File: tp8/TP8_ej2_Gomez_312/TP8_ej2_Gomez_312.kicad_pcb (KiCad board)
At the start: 2 copper layers, 50 x 40 mm, 32 parts, among them J1 Output - RL, J10 Vemisor, J11 Vemisor, J2 Power, J3 Input, J5 GND, J6 Vbase, J7 Vbase, J8 Vbase, J9 Vemisor, Q1 BC548C, Q2 BC547, Q3 BC548C

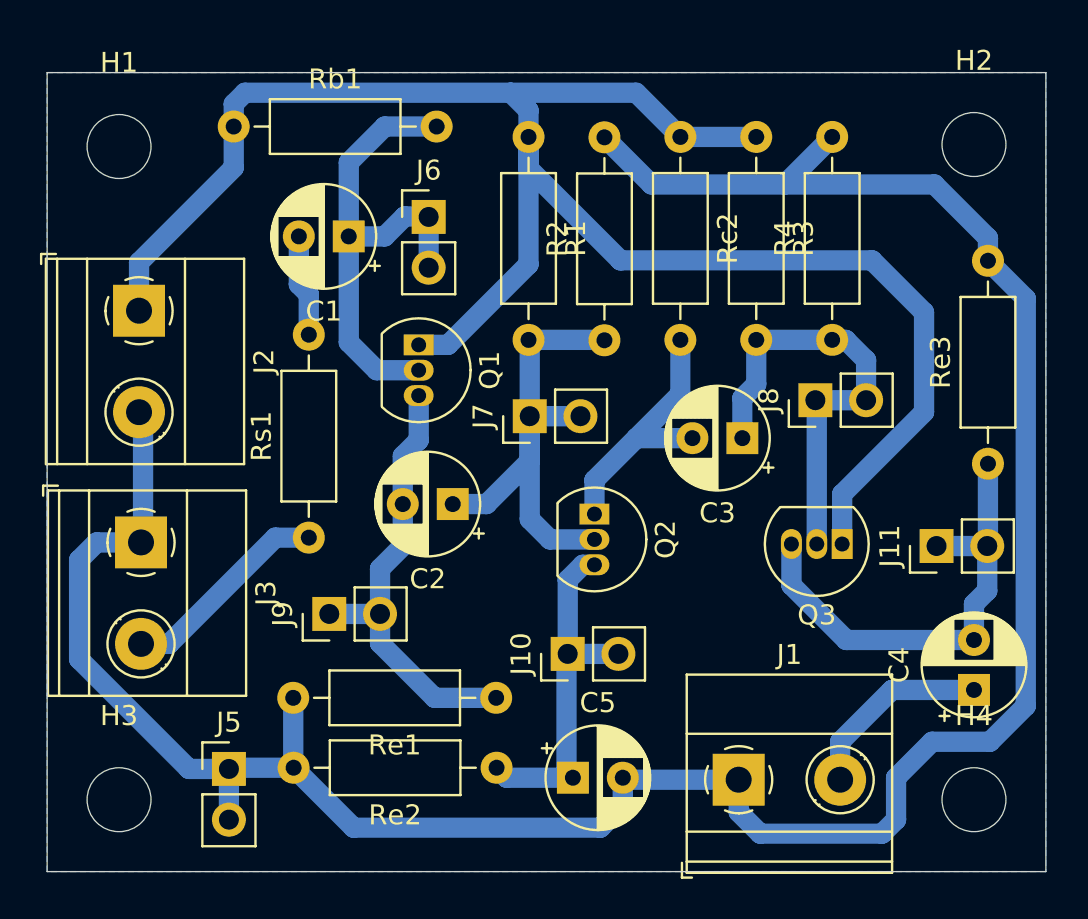
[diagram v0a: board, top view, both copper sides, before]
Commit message: finish tp8
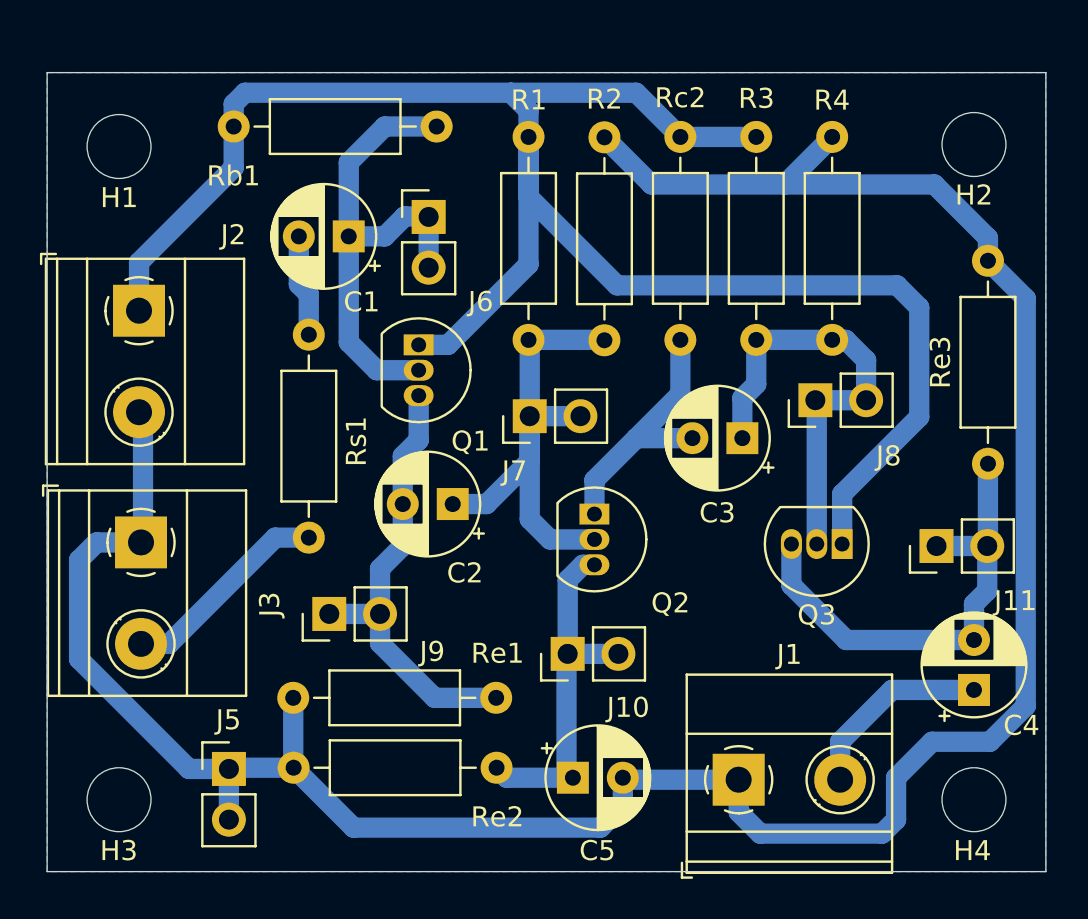
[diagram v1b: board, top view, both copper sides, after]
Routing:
- net VCC: track 93.4 -> 94.0 mm
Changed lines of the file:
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@@
 			(sketchpadsonfab no)
 			(subtractmaskfromsilk no)
-			(outputformat 1)
-			(mirror no)
-			(drillshape 1)
+			(outputformat 4)
+			(mirror yes)
+			(drillshape 0)
 			(scaleselection 1)
 			(outputdirectory "")
@@
 		(tags "Through hole pin header THT 1x02 2.54mm single row")
 		(property "Reference" "J7"
-			(at 0 -2.33 -90)
+			(at -2.75 -0.76 0)
 			(layer "F.SilkS")
 			(effects
@@
 		(tags "Through hole pin header THT 1x02 2.54mm single row")
 		(property "Reference" "J8"
-			(at 0 -2.33 270)
+			(at -2.8 3.67 0)
 			(layer "F.SilkS")
 			(effects
@@
 		)
 		(property "Value" "Vbase"
-			(at 0 4.87 270)
+			(at 0 4.87 -90)
 			(layer "F.Fab")
 			(effects
@@
 		)
 		(fp_text user "${REFERENCE}"
-			(at 0 1.27 360)
+			(at 0 1.27 0)
 			(layer "F.Fab")
 			(effects
@@
 		(tags "Resistor Axial_DIN0207 series Axial Horizontal pin pitch 10.16mm 0.25W = 1/4W length 6.3mm diameter 2.5mm")
 		(property "Reference" "R2"
-			(at 5.08 -2.37 -90)
+			(at 12.06 0 0)
 			(layer "F.SilkS")
 			(effects
@@
 		(tags "Resistor Axial_DIN0207 series Axial Horizontal pin pitch 10.16mm 0.25W = 1/4W length 6.3mm diameter 2.5mm")
 		(property "Reference" "Rs1"
-			(at 5.08 -2.37 -90)
+			(at 4.82 2.39 -90)
 			(layer "F.SilkS")
 			(effects
@@
 		(tags "Through hole pin header THT 1x02 2.54mm single row")
 		(property "Reference" "J11"
-			(at 0 -2.33 -90)
+			(at -2.75 3.955 0)
 			(layer "F.SilkS")
 			(effects
@@
 		(tags "Through hole pin header THT 1x02 2.54mm single row")
 		(property "Reference" "J10"
-			(at 0 -2.33 -90)
+			(at -2.69 3.03 0)
 			(layer "F.SilkS")
 			(effects
@@
 		(tags "Through hole pin header THT 1x02 2.54mm single row")
 		(property "Reference" "J9"
-			(at 0 -2.33 -90)
+			(at -1.89 5.155 0)
 			(layer "F.SilkS")
 			(effects
@@
 		(tags "mounting hole 3.2mm no annular m3")
 		(property "Reference" "H4"
-			(at 0 -4.2 0)
+			(at -0.08 2.56 0)
 			(layer "F.SilkS")
 			(effects
@@
 		(tags "Resistor Axial_DIN0207 series Axial Horizontal pin pitch 10.16mm 0.25W = 1/4W length 6.3mm diameter 2.5mm")
 		(property "Reference" "Rc2"
-			(at 5.08 -2.37 90)
+			(at -1.95 0 180)
 			(layer "F.SilkS")
 			(effects
@@
 		(tags "CP Radial series Radial pin pitch 2.50mm  diameter 5mm Electrolytic Capacitor")
 		(property "Reference" "C2"
-			(at 1.25 -3.75 180)
+			(at -0.614887 -3.46 180)
 			(layer "F.SilkS")
 			(effects
@@
 		(tags "THT Terminal Block Phoenix MKDS-1,5-2-5.08 pitch 5.08mm size 10.2x9.8mm^2 drill 1.3mm pad 2.6mm")
 		(property "Reference" "J3"
-			(at 2.54 -6.26 -90)
+			(at 3.1 -6.45 -90)
 			(layer "F.SilkS")
 			(effects
@@
 		(tags "Resistor Axial_DIN0207 series Axial Horizontal pin pitch 10.16mm 0.25W = 1/4W length 6.3mm diameter 2.5mm")
 		(property "Reference" "R3"
-			(at 5.08 -2.37 90)
+			(at -1.92 -0.01 180)
 			(layer "F.SilkS")
 			(effects
@@
 		(tags "to-92 sc-43 sc-43a sot54 PA33 transistor")
 		(property "Reference" "Q2"
-			(at 1.27 -3.56 90)
+			(at 4.46 -3.81 180)
 			(layer "F.SilkS")
 			(effects
@@
 		(tags "Resistor Axial_DIN0207 series Axial Horizontal pin pitch 10.16mm 0.25W = 1/4W length 6.3mm diameter 2.5mm")
 		(property "Reference" "Re2"
-			(at 5.08 -2.37 180)
+			(at -0.04 -2.47 180)
 			(layer "F.SilkS")
 			(effects
@@
 		(tags "Through hole pin header THT 1x02 2.54mm single row")
 		(property "Reference" "J6"
-			(at 0 -2.33 0)
+			(at 2.61 4.245 0)
 			(layer "F.SilkS")
 			(effects
@@
 		(tags "to-92 sc-43 sc-43a sot54 PA33 transistor")
 		(property "Reference" "Q1"
-			(at 1.27 -3.56 90)
+			(at 4.83 -2.6 180)
 			(layer "F.SilkS")
 			(effects
@@
 		(tags "Through hole pin header THT 1x02 2.54mm single row")
 		(property "Reference" "J5"
-			(at 0 -2.33 0)
+			(at -0.02 -2.45 0)
 			(layer "F.SilkS")
 			(effects
@@
 		(tags "Resistor Axial_DIN0207 series Axial Horizontal pin pitch 10.16mm 0.25W = 1/4W length 6.3mm diameter 2.5mm")
 		(property "Reference" "Rb1"
-			(at 5.08 -2.37 0)
+			(at -0.01 2.48 0)
 			(layer "F.SilkS")
 			(effects
@@
 		(tags "Resistor Axial_DIN0207 series Axial Horizontal pin pitch 10.16mm 0.25W = 1/4W length 6.3mm diameter 2.5mm")
 		(property "Reference" "R1"
-			(at 5.08 -2.37 90)
+			(at -1.84 -0.02 180)
 			(layer "F.SilkS")
 			(effects
@@
 		(tags "mounting hole 3.2mm no annular m3")
 		(property "Reference" "H1"
-			(at 0 -4.2 0)
+			(at 0.01 2.57 0)
 			(layer "F.SilkS")
 			(effects
@@
 		(tags "THT Terminal Block Phoenix MKDS-1,5-2-5.08 pitch 5.08mm size 10.2x9.8mm^2 drill 1.3mm pad 2.6mm")
 		(property "Reference" "J2"
-			(at 2.54 -6.26 -90)
+			(at -3.79 -4.72 0)
 			(layer "F.SilkS")
 			(effects
@@
 		(tags "Resistor Axial_DIN0207 series Axial Horizontal pin pitch 10.16mm 0.25W = 1/4W length 6.3mm diameter 2.5mm")
 		(property "Reference" "R4"
-			(at 5.08 -2.37 -90)
+			(at 11.99 -0.01 0)
 			(layer "F.SilkS")
 			(effects
@@
 		(tags "CP Radial series Radial pin pitch 2.50mm  diameter 5mm Electrolytic Capacitor")
 		(property "Reference" "C1"
-			(at 1.25 -3.75 180)
+			(at -0.65 -3.29 180)
 			(layer "F.SilkS")
 			(effects
@@
 		(tags "mounting hole 3.2mm no annular m3")
 		(property "Reference" "H2"
-			(at 0 -4.2 0)
+			(at 0 2.54 0)
 			(layer "F.SilkS")
 			(effects
@@
 		(tags "Resistor Axial_DIN0207 series Axial Horizontal pin pitch 10.16mm 0.25W = 1/4W length 6.3mm diameter 2.5mm")
 		(property "Reference" "Re1"
-			(at 5.08 -2.37 180)
+			(at -0.07 2.22 180)
 			(layer "F.SilkS")
 			(effects
@@
 		(tags "CP Radial series Radial pin pitch 2.50mm  diameter 5mm Electrolytic Capacitor")
 		(property "Reference" "C4"
-			(at 1.25 -3.75 -90)
+			(at -1.784887 2.38 0)
 			(layer "F.SilkS")
 			(effects
@@
 		(tags "mounting hole 3.2mm no annular m3")
 		(property "Reference" "H3"
-			(at 0 -4.2 0)
+			(at -0.01 2.56 0)
 			(layer "F.SilkS")
 			(effects
@@
 		(tags "CP Radial series Radial pin pitch 2.50mm  diameter 5mm Electrolytic Capacitor")
 		(property "Reference" "C5"
-			(at 1.25 -3.75 0)
+			(at 1.23 3.66 0)
 			(layer "F.SilkS")
 			(effects
@@
 	)
 	(segment
-		(start 24.6 31.92)
-		(end 24.6 29.5)
-		(width 1.016)
-		(layer "B.Cu")
-		(net 11)
-	)
-	(segment
-		(start 61.3 29.4)
-		(end 48.7 29.4)
+		(start 44.1 26.22)
+		(end 44.1 23.22)
 		(width 1.016)
 		(layer "B.Cu")
@@
 	)
 	(segment
-		(start 48.7 29.4)
-		(end 44.1 24.8)
+		(start 24.6 31.92)
+		(end 24.6 29.5)
 		(width 1.016)
 		(layer "B.Cu")
@@
 	)
 	(segment
-		(start 63.9 37)
-		(end 63.9 32)
+		(start 63.66 37.24)
+		(end 63.66 31.76)
 		(width 1.016)
 		(layer "B.Cu")
@@
 	)
 	(segment
-		(start 59.8 41.1)
-		(end 63.9 37)
-		(width 1.016)
-		(layer "B.Cu")
-		(net 11)
-	)
-	(segment
-		(start 44.1 24.8)
-		(end 44.1 23.22)
+		(start 59.8 43.6)
+		(end 59.8 41.1)
 		(width 1.016)
 		(layer "B.Cu")
@@
 	)
 	(segment
-		(start 63.9 32)
-		(end 61.3 29.4)
+		(start 62.55 30.65)
+		(end 48.53 30.65)
 		(width 1.016)
 		(layer "B.Cu")
@@
 	)
 	(segment
-		(start 59.8 43.6)
-		(end 59.8 41.1)
-		(width 1.016)
-		(layer "B.Cu")
-		(net 11)
-	)
-	(segment
 		(start 29.9 21.008)
 		(end 43.208 21.008)
@@
 	)
 	(segment
+		(start 63.66 31.76)
+		(end 62.55 30.65)
+		(width 1.016)
+		(layer "B.Cu")
+		(net 11)
+	)
+	(segment
 		(start 29.34 21.568)
 		(end 29.9 21.008)
 		(width 1.016)
 		(layer "B.Cu")
+		(net 11)
+	)
+	(segment
+		(start 48.53 30.65)
+		(end 44.1 26.22)
+		(width 1.016)
+		(layer "B.Cu")
+		(net 11)
+	)
+	(segment
+		(start 59.8 41.1)
+		(end 63.66 37.24)
+		(width 1.016)
+		(layer "B.Cu")
